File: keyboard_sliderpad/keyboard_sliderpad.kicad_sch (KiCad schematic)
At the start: 13 parts, among them J1 Conn_01x04_Pin, J2 Conn_01x04_Pin, J3 Conn_01x04_Pin, J4 Conn_01x04_Pin, SW1 RotaryEncoder_Switch, SW2 RotaryEncoder_Switch, U1 XIAO-RP2040-DIP

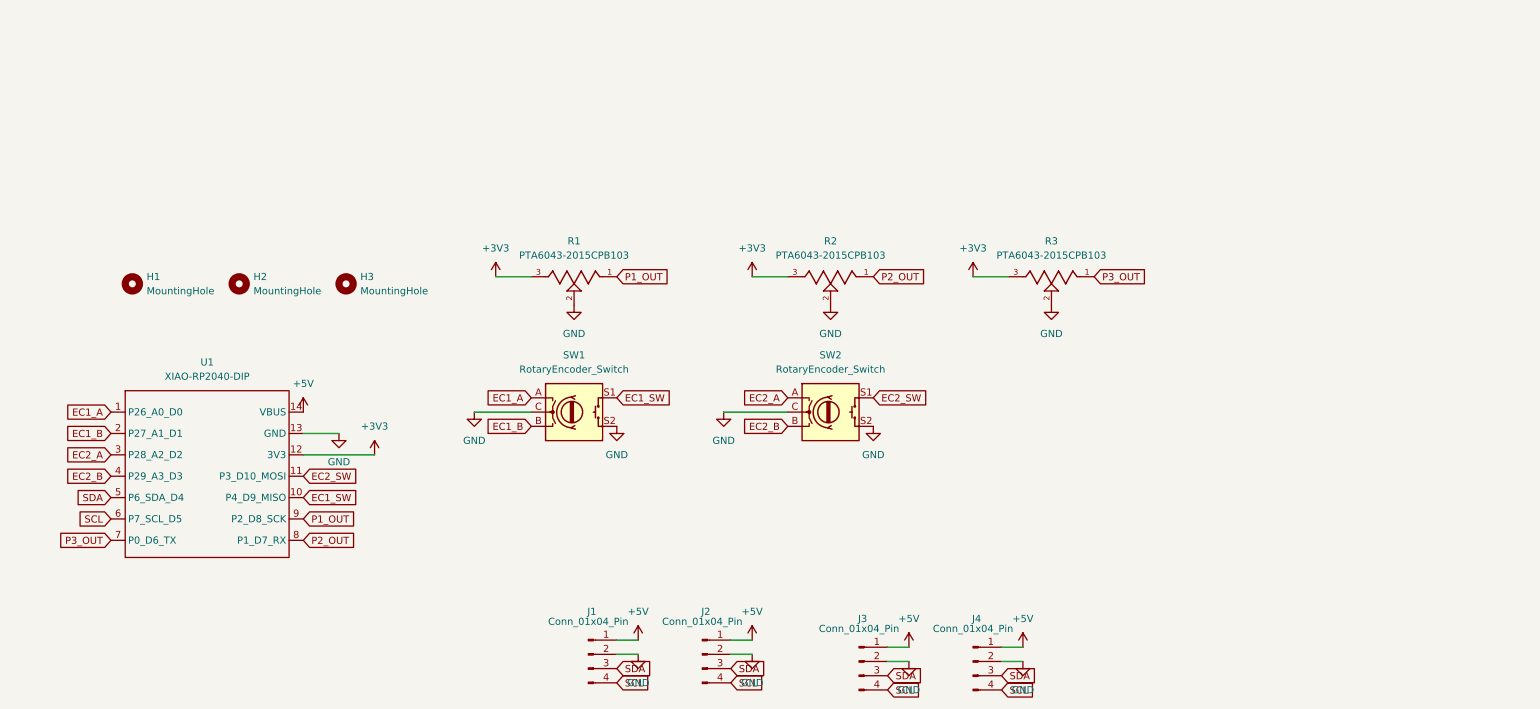
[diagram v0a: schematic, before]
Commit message: updates
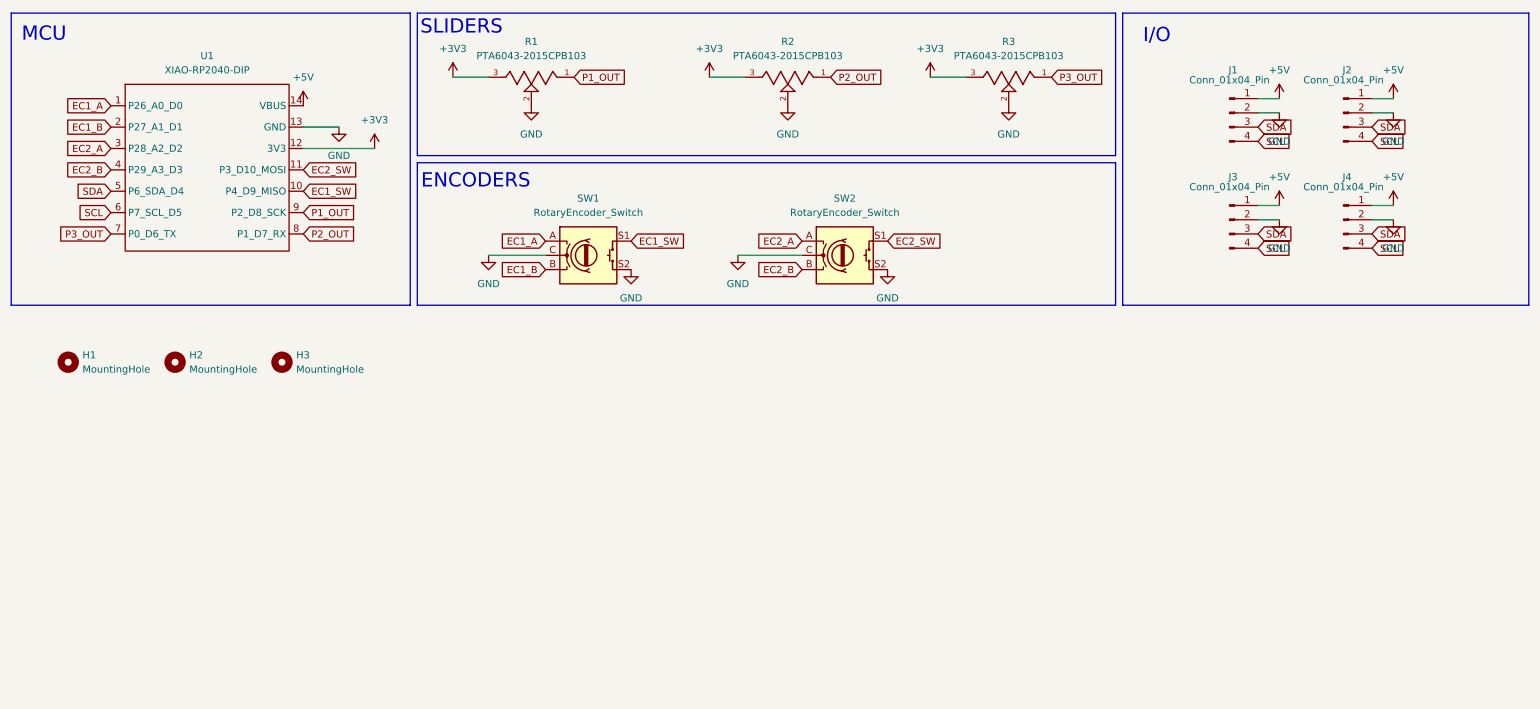
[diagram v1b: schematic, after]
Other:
- note added: "ENCODERS"
- note added: "I/O"
- note added: "MCU"
- note added: "SLIDERS"
- moved on the sheet: H1, H2, H3, J1, J2, J3, J4, R1, R2, R3, SW1, SW2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
